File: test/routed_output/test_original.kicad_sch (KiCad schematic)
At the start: 6 parts, among them U1 R_0805_2012Metric_Pad1.20x1.4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, U2 SOT-23, U3 TO-220-3_Horizontal_TabDown, U4 TO-92_Wide, U5 R_Axial_DIN0207_L6.3mm_D2.5mm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, U6 R_Axial_DIN0207_L6.3mm_D2.5mm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

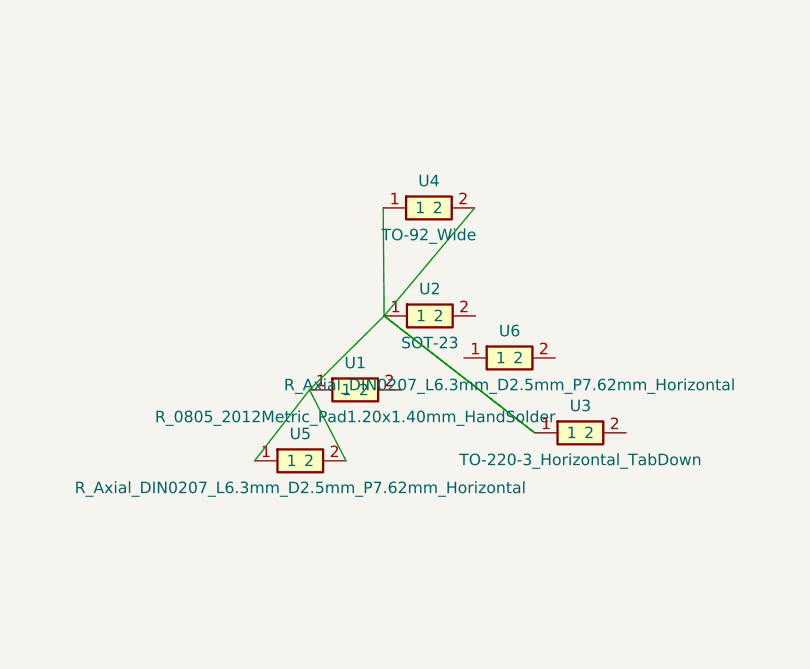
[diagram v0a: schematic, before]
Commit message: backup
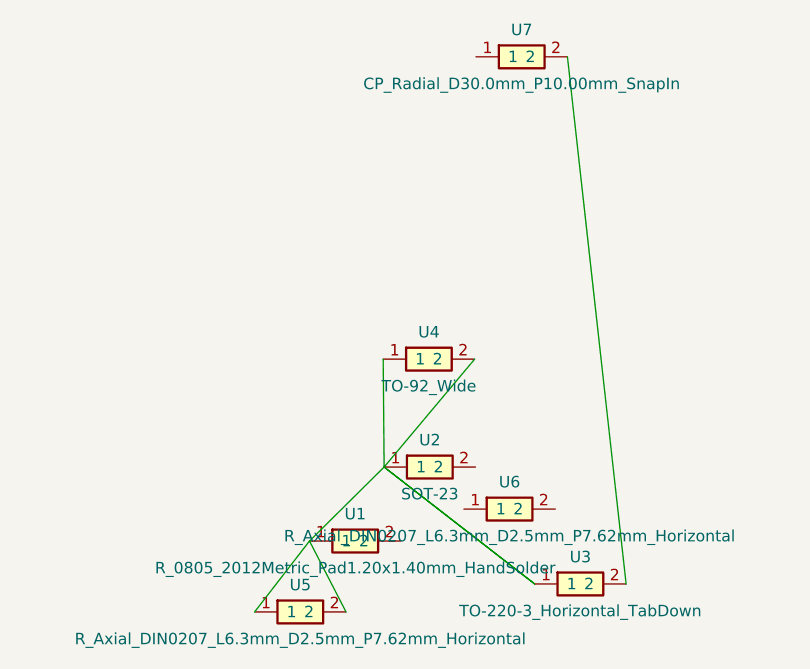
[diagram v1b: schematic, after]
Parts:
- added U7: CP_Radial_D30.0mm_P10.00mm_SnapIn, RE_passive_tht:CP_Radial_D30.0mm_P10.00mm_SnapIn, symbol RE_passive:C_Polarized
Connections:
- net at U3.2: now also U7.2
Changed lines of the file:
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@@
   (symbol
     (lib_id "RE_passive:R")
-    (at 139.04 111.17 0)
-    (unit 1)
-    (exclude_from_sim no)
-    (in_bom yes)
-    (on_board yes)
-    (dnp no)
-    (property "Reference" "U1" (at 139.04 108.17 0)
-      (effects (font (size 1.27 1.27)))
-    )
-    (property "Value" "R_0805_2012Metric_Pad1.20x1.40mm_HandSolder" (at 139.04 114.17 0)
-      (effects (font (size 1.27 1.27)))
-    )
-    (property "Footprint" "00_basic:R_0805_2012Metric_Pad1.20x1.40mm_HandSolder" (at 139.04 116.17 0)
-      (effects (font (size 1.27 1.27)) hide)
-    )
-    (instances
-      (project ""
-        (path "/"
+    (at 139.04 127.96 0)
+    (unit 1)
+    (exclude_from_sim no)
+    (in_bom yes)
+    (on_board yes)
+    (dnp no)
+    (property "Reference" "U1" (at 139.04 124.96 0)
+      (effects (font (size 1.27 1.27)))
+    )
+    (property "Value" "R_0805_2012Metric_Pad1.20x1.40mm_HandSolder" (at 139.04 130.96 0)
+      (effects (font (size 1.27 1.27)))
+    )
+    (property "Footprint" "00_basic:R_0805_2012Metric_Pad1.20x1.40mm_HandSolder" (at 139.04 132.96 0)
+      (effects (font (size 1.27 1.27)) hide)
+    )
+    (instances
+      (project ""
+        (path "/76b0d100-f5a4-4cb0-a1b7-3defec0bed4b"
           (reference "U1")
           (unit 1)
@@
   (symbol
     (lib_id "RE_active:Q_NPN")
-    (at 147.33 102.95 0)
-    (unit 1)
-    (exclude_from_sim no)
-    (in_bom yes)
-    (on_board yes)
-    (dnp no)
-    (property "Reference" "U2" (at 147.33 99.95 0)
-      (effects (font (size 1.27 1.27)))
-    )
-    (property "Value" "SOT-23" (at 147.33 105.95 0)
-      (effects (font (size 1.27 1.27)))
-    )
-    (property "Footprint" "RE_active:SOT-23" (at 147.33 107.95 0)
-      (effects (font (size 1.27 1.27)) hide)
-    )
-    (instances
-      (project ""
-        (path "/"
+    (at 147.33 119.74 0)
+    (unit 1)
+    (exclude_from_sim no)
+    (in_bom yes)
+    (on_board yes)
+    (dnp no)
+    (property "Reference" "U2" (at 147.33 116.74 0)
+      (effects (font (size 1.27 1.27)))
+    )
+    (property "Value" "SOT-23" (at 147.33 122.74 0)
+      (effects (font (size 1.27 1.27)))
+    )
+    (property "Footprint" "RE_active:SOT-23" (at 147.33 124.74 0)
+      (effects (font (size 1.27 1.27)) hide)
+    )
+    (instances
+      (project ""
+        (path "/76b0d100-f5a4-4cb0-a1b7-3defec0bed4b"
           (reference "U2")
           (unit 1)
@@
   (symbol
     (lib_id "RE_active:Q_NMOS")
-    (at 164.06 115.94 0)
-    (unit 1)
-    (exclude_from_sim no)
-    (in_bom yes)
-    (on_board yes)
-    (dnp no)
-    (property "Reference" "U3" (at 164.06 112.94 0)
-      (effects (font (size 1.27 1.27)))
-    )
-    (property "Value" "TO-220-3_Horizontal_TabDown" (at 164.06 118.94 0)
-      (effects (font (size 1.27 1.27)))
-    )
-    (property "Footprint" "RE_active:TO-220-3_Horizontal_TabDown" (at 164.06 120.94 0)
-      (effects (font (size 1.27 1.27)) hide)
-    )
-    (instances
-      (project ""
-        (path "/"
+    (at 164.06 132.73 0)
+    (unit 1)
+    (exclude_from_sim no)
+    (in_bom yes)
+    (on_board yes)
+    (dnp no)
+    (property "Reference" "U3" (at 164.06 129.73 0)
+      (effects (font (size 1.27 1.27)))
+    )
+    (property "Value" "TO-220-3_Horizontal_TabDown" (at 164.06 135.73 0)
+      (effects (font (size 1.27 1.27)))
+    )
+    (property "Footprint" "RE_active:TO-220-3_Horizontal_TabDown" (at 164.06 137.73 0)
+      (effects (font (size 1.27 1.27)) hide)
+    )
+    (instances
+      (project ""
+        (path "/76b0d100-f5a4-4cb0-a1b7-3defec0bed4b"
           (reference "U3")
           (unit 1)
@@
   (symbol
     (lib_id "RE_active:Q_NPN")
-    (at 147.23 90.95 0)
-    (unit 1)
-    (exclude_from_sim no)
-    (in_bom yes)
-    (on_board yes)
-    (dnp no)
-    (property "Reference" "U4" (at 147.23 87.95 0)
-      (effects (font (size 1.27 1.27)))
-    )
-    (property "Value" "TO-92_Wide" (at 147.23 93.95 0)
-      (effects (font (size 1.27 1.27)))
-    )
-    (property "Footprint" "RE_active:TO-92_Wide" (at 147.23 95.95 0)
-      (effects (font (size 1.27 1.27)) hide)
-    )
-    (instances
-      (project ""
-        (path "/"
+    (at 147.23 107.75 0)
+    (unit 1)
+    (exclude_from_sim no)
+    (in_bom yes)
+    (on_board yes)
+    (dnp no)
+    (property "Reference" "U4" (at 147.23 104.75 0)
+      (effects (font (size 1.27 1.27)))
+    )
+    (property "Value" "TO-92_Wide" (at 147.23 110.75 0)
+      (effects (font (size 1.27 1.27)))
+    )
+    (property "Footprint" "RE_active:TO-92_Wide" (at 147.23 112.75 0)
+      (effects (font (size 1.27 1.27)) hide)
+    )
+    (instances
+      (project ""
+        (path "/76b0d100-f5a4-4cb0-a1b7-3defec0bed4b"
           (reference "U4")
           (unit 1)
@@
   (symbol
     (lib_id "_placeholder:U5")
-    (at 132.94 119.05 0)
-    (unit 1)
-    (exclude_from_sim no)
-    (in_bom yes)
-    (on_board yes)
-    (dnp no)
-    (property "Reference" "U5" (at 132.94 116.05 0)
-      (effects (font (size 1.27 1.27)))
-    )
-    (property "Value" "R_Axial_DIN0207_L6.3mm_D2.5mm_P7.62mm_Horizontal" (at 132.94 122.05 0)
-      (effects (font (size 1.27 1.27)))
-    )
-    (property "Footprint" "RE_passive_tht:R_Axial_DIN0207_L6.3mm_D2.5mm_P7.62mm_Horizontal" (at 132.94 124.05 0)
-      (effects (font (size 1.27 1.27)) hide)
-    )
-    (instances
-      (project ""
-        (path "/"
+    (at 132.94 135.84 0)
+    (unit 1)
+    (exclude_from_sim no)
+    (in_bom yes)
+    (on_board yes)
+    (dnp no)
+    (property "Reference" "U5" (at 132.94 132.84 0)
+      (effects (font (size 1.27 1.27)))
+    )
+    (property "Value" "R_Axial_DIN0207_L6.3mm_D2.5mm_P7.62mm_Horizontal" (at 132.94 138.84 0)
+      (effects (font (size 1.27 1.27)))
+    )
+    (property "Footprint" "RE_passive_tht:R_Axial_DIN0207_L6.3mm_D2.5mm_P7.62mm_Horizontal" (at 132.94 140.84 0)
+      (effects (font (size 1.27 1.27)) hide)
+    )
+    (instances
+      (project ""
+        (path "/76b0d100-f5a4-4cb0-a1b7-3defec0bed4b"
           (reference "U5")
           (unit 1)
@@
   (symbol
     (lib_id "_placeholder:U6")
-    (at 156.19 107.62 0)
-    (unit 1)
-    (exclude_from_sim no)
-    (in_bom yes)
-    (on_board yes)
-    (dnp no)
-    (property "Reference" "U6" (at 156.19 104.62 0)
-      (effects (font (size 1.27 1.27)))
-    )
-    (property "Value" "R_Axial_DIN0207_L6.3mm_D2.5mm_P7.62mm_Horizontal" (at 156.19 110.62 0)
-      (effects (font (size 1.27 1.27)))
-    )
-    (property "Footprint" "RE_passive_tht:R_Axial_DIN0207_L6.3mm_D2.5mm_P7.62mm_Horizontal" (at 156.19 112.62 0)
-      (effects (font (size 1.27 1.27)) hide)
-    )
-    (instances
-      (project ""
-        (path "/"
+    (at 156.19 124.41 0)
+    (unit 1)
+    (exclude_from_sim no)
+    (in_bom yes)
+    (on_board yes)
+    (dnp no)
+    (property "Reference" "U6" (at 156.19 121.41 0)
+      (effects (font (size 1.27 1.27)))
+    )
+    (property "Value" "R_Axial_DIN0207_L6.3mm_D2.5mm_P7.62mm_Horizontal" (at 156.19 127.41 0)
+      (effects (font (size 1.27 1.27)))
+    )
+    (property "Footprint" "RE_passive_tht:R_Axial_DIN0207_L6.3mm_D2.5mm_P7.62mm_Horizontal" (at 156.19 129.41 0)
+      (effects (font (size 1.27 1.27)) hide)
+    )
+    (instances
+      (project ""
+        (path "/76b0d100-f5a4-4cb0-a1b7-3defec0bed4b"
           (reference "U6")
           (unit 1)
@@
     )
   )
-  (wire (pts (xy 152.31 90.95) (xy 142.25 102.95))
-    (stroke (width 0) (type default))
-  )
-  (wire (pts (xy 142.25 102.95) (xy 158.98 115.94))
-    (stroke (width 0) (type default))
-  )
-  (wire (pts (xy 142.25 102.95) (xy 158.98 115.94))
-    (stroke (width 0) (type default))
-  )
-  (wire (pts (xy 142.25 102.95) (xy 142.15 90.95))
-    (stroke (width 0) (type default))
-  )
-  (wire (pts (xy 133.96 111.17) (xy 142.25 102.95))
-    (stroke (width 0) (type default))
-  )
-  (wire (pts (xy 133.96 111.17) (xy 127.86 119.05))
-    (stroke (width 0) (type default))
-  )
-  (wire (pts (xy 133.96 111.17) (xy 138.02 119.05))
-    (stroke (width 0) (type default))
-  )
+  (symbol
+    (lib_id "RE_passive:C_Polarized")
+    (at 157.54 74.16 0)
+    (unit 1)
+    (exclude_from_sim no)
+    (in_bom yes)
+    (on_board yes)
+    (dnp no)
+    (property "Reference" "U7" (at 157.54 71.16 0)
+      (effects (font (size 1.27 1.27)))
+    )
+    (property "Value" "CP_Radial_D30.0mm_P10.00mm_SnapIn" (at 157.54 77.16 0)
+      (effects (font (size 1.27 1.27)))
+    )
+    (property "Footprint" "RE_passive_tht:CP_Radial_D30.0mm_P10.00mm_SnapIn" (at 157.54 79.16 0)
+      (effects (font (size 1.27 1.27)) hide)
+    )
+    (instances
+      (project ""
+        (path "/76b0d100-f5a4-4cb0-a1b7-3defec0bed4b"
+          (reference "U7")
+          (unit 1)
+        )
+      )
+    )
+  )
+  (wire (pts (xy 152.31 107.75) (xy 142.25 119.74))
+    (stroke (width 0) (type default))
+  )
+  (wire (pts (xy 142.25 119.74) (xy 158.98 132.73))
+    (stroke (width 0) (type default))
+  )
+  (wire (pts (xy 142.25 119.74) (xy 158.98 132.73))
+    (stroke (width 0) (type default))
+  )
+  (wire (pts (xy 142.25 119.74) (xy 142.15 107.75))
+    (stroke (width 0) (type default))
+  )
+  (wire (pts (xy 133.96 127.96) (xy 142.25 119.74))
+    (stroke (width 0) (type default))
+  )
+  (wire (pts (xy 133.96 127.96) (xy 127.86 135.84))
+    (stroke (width 0) (type default))
+  )
+  (wire (pts (xy 133.96 127.96) (xy 138.02 135.84))
+    (stroke (width 0) (type default))
+  )
+  (wire (pts (xy 169.14 132.73) (xy 162.62 74.16))
+    (stroke (width 0) (type default))
+  )
